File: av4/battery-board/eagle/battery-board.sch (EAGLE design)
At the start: 66 parts, among them J100 ROCKETNET-BATTERY-14, J101 87758-0216, J102 87758-0216, Q100 Si2343DS-T1, Q101 SI4435DDY, Q102 SI4435DDY, Q103 SI1023X, Q104 SI1023X, U100 BQ3060PW

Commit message: Latest battery boards notes, handing off to Michael for final polishing.
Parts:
- C101, C102, C105, C109, C111, C112, C113, C114: device rcl_custom:C-EU0402-B-NOSILK -> rcl_custom:C-EU0603-B-NOSILK
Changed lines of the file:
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@@
 <setting verticaltext="up"/>
 </settings>
-<grid distance="0.05" unitdist="inch" unit="inch" style="lines" multiple="2" display="yes" altdistance="0.01" altunitdist="inch" altunit="inch"/>
+<grid distance="0.1" unitdist="inch" unit="inch" style="lines" multiple="1" display="no" altdistance="0.01" altunitdist="inch" altunit="inch"/>
 <layers>
 <layer number="1" name="Top" color="4" fill="1" visible="no" active="no"/>
@@
 <part name="R120" library="rcl_custom" deviceset="R-US_" device="0603-B-NOSILK" value="100"/>
 <part name="R121" library="rcl_custom" deviceset="R-US_" device="0603-B-NOSILK" value="100"/>
-<part name="C111" library="rcl_custom" deviceset="C-EU" device="0402-B-NOSILK" value="100n"/>
-<part name="C113" library="rcl_custom" deviceset="C-EU" device="0402-B-NOSILK" value="100n"/>
-<part name="C112" library="rcl_custom" deviceset="C-EU" device="0402-B-NOSILK" value="100n"/>
+<part name="C111" library="rcl_custom" deviceset="C-EU" device="0603-B-NOSILK" value="100n"/>
+<part name="C113" library="rcl_custom" deviceset="C-EU" device="0603-B-NOSILK" value="100n"/>
+<part name="C112" library="rcl_custom" deviceset="C-EU" device="0603-B-NOSILK" value="100n"/>
 <part name="BAR_GND4" library="psas" deviceset="SUP_GND_BAR" device=""/>
 <part name="BAR_GND6" library="psas" deviceset="SUP_GND_BAR" device=""/>
@@
 <part name="R111" library="rcl_custom" deviceset="R-US_" device="0603-B-NOSILK" value="1K"/>
 <part name="R119" library="rcl_custom" deviceset="R-US_" device="0603-B-NOSILK" value="1K"/>
-<part name="C101" library="rcl_custom" deviceset="C-EU" device="0402-B-NOSILK" value="100n"/>
-<part name="C102" library="rcl_custom" deviceset="C-EU" device="0402-B-NOSILK" value="100n"/>
-<part name="C105" library="rcl_custom" deviceset="C-EU" device="0402-B-NOSILK" value="100n"/>
-<part name="C114" library="rcl_custom" deviceset="C-EU" device="0402-B-NOSILK" value="100n"/>
+<part name="C101" library="rcl_custom" deviceset="C-EU" device="0603-B-NOSILK" value="100n"/>
+<part name="C102" library="rcl_custom" deviceset="C-EU" device="0603-B-NOSILK" value="100n"/>
+<part name="C105" library="rcl_custom" deviceset="C-EU" device="0603-B-NOSILK" value="100n"/>
+<part name="C114" library="rcl_custom" deviceset="C-EU" device="0603-B-NOSILK" value="100n"/>
 <part name="BAR_GND8" library="psas" deviceset="SUP_GND_BAR" device=""/>
 <part name="BAR_GND9" library="psas" deviceset="SUP_GND_BAR" device=""/>
@@
 <part name="BAR_GND11" library="psas" deviceset="SUP_GND_BAR" device=""/>
 <part name="BAR_GND12" library="psas" deviceset="SUP_GND_BAR" device=""/>
-<part name="C109" library="rcl_custom" deviceset="C-EU" device="0402-B-NOSILK" value="100n"/>
+<part name="C109" library="rcl_custom" deviceset="C-EU" device="0603-B-NOSILK" value="100n"/>
 <part name="C110" library="rcl_custom" deviceset="C-EU" device="0603-B-NOSILK" value="1u"/>
 <part name="D101" library="diode-0603" deviceset="DIODE-0603" device=""/>

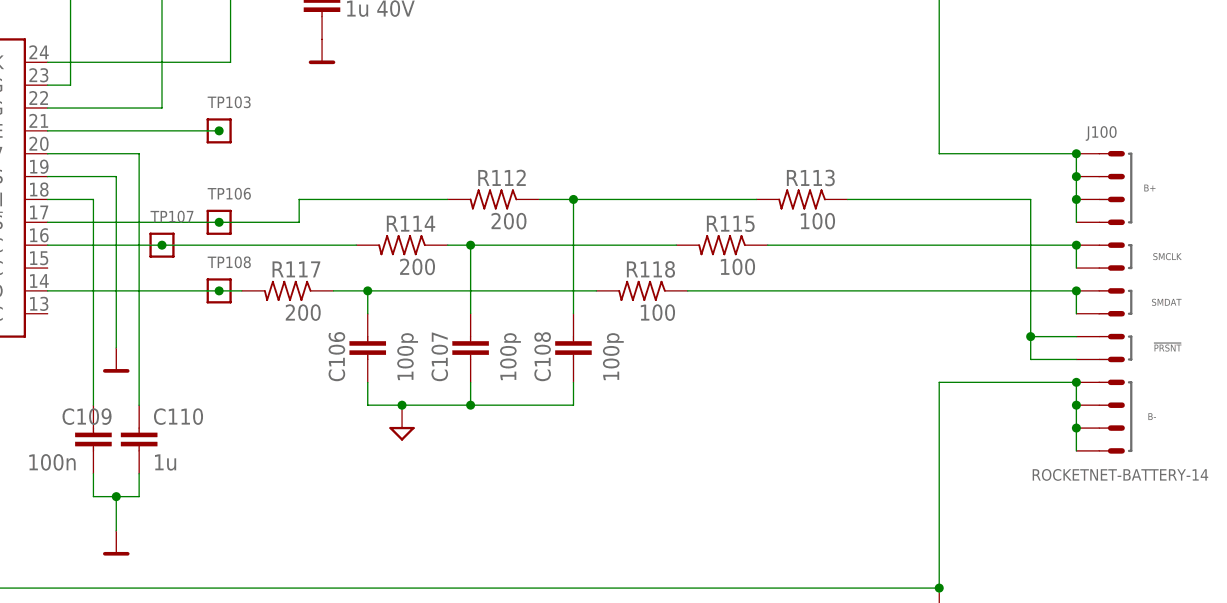
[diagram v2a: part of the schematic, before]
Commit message: moved some routing to top layer, needs drc work
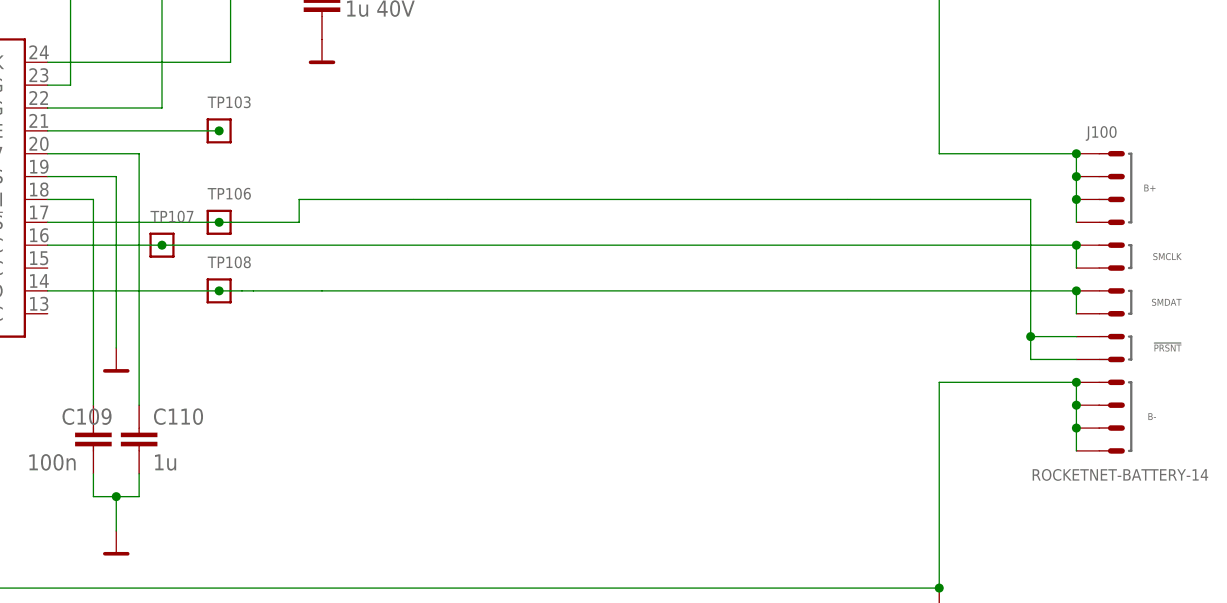
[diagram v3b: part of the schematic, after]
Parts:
- removed C106, C107, C108: 100p, rcl_custom:C-EU0603-B-NOSILK
- removed R112, R114, R117: 200, rcl_custom:R-US_0603-B-NOSILK
- removed R113, R115, R118: 100, rcl_custom:R-US_0603-B-NOSILK
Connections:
- removed net N$17: C106.1, R117.1, R118.2
- removed net N$24: C107.1, R114.1, R115.2
- removed net N$33: C108.1, R112.1, R113.2
- removed net RNC-!PRSNT: J100.!PRSNT@1, J100.!PRSNT@2, R113.1
- removed net RNC-SDAT: J100.SMDAT@1, J100.SMDAT@2, R118.1
- removed net SMBC: R114.2, TP107.P$1, U100.SMBC
- net !PRES: now also J100.!PRSNT@1, J100.!PRSNT@2; no longer R112.2
- net RNC-SCLK: now also TP107.P$1, U100.SMBC; no longer R115.1
- net SMBD: now also J100.SMDAT@1, J100.SMDAT@2; no longer R117.2
- net TRIANGLE_GND: no longer C106.2, C107.2, C108.2
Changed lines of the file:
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@@
 <part name="R110" library="rcl_custom" deviceset="R-US_" device="0603-B-NOSILK" value="100 .25W"/>
 <part name="R105" library="rcl_custom" deviceset="R-US_" device="0603-B-NOSILK" value="100 .25W"/>
-<part name="R114" library="rcl_custom" deviceset="R-US_" device="0603-B-NOSILK" value="200"/>
-<part name="R115" library="rcl_custom" deviceset="R-US_" device="0603-B-NOSILK" value="100"/>
-<part name="R117" library="rcl_custom" deviceset="R-US_" device="0603-B-NOSILK" value="200"/>
-<part name="R118" library="rcl_custom" deviceset="R-US_" device="0603-B-NOSILK" value="100"/>
-<part name="C106" library="rcl_custom" deviceset="C-EU" device="0603-B-NOSILK" value="100p"/>
-<part name="TRIANGLE_GND1" library="psas" deviceset="SUP_GND_TRIANGLE" device=""/>
-<part name="C107" library="rcl_custom" deviceset="C-EU" device="0603-B-NOSILK" value="100p"/>
 <part name="D102" library="diode-0603" deviceset="DIODE-0603" device=""/>
 <part name="C104" library="rcl_custom" deviceset="C-EU" device="0603-B-NOSILK" value="1u 40V"/>
 <part name="BAR_GND14" library="psas" deviceset="SUP_GND_BAR" device=""/>
-<part name="R112" library="rcl_custom" deviceset="R-US_" device="0603-B-NOSILK" value="200"/>
-<part name="R113" library="rcl_custom" deviceset="R-US_" device="0603-B-NOSILK" value="100"/>
-<part name="C108" library="rcl_custom" deviceset="C-EU" device="0603-B-NOSILK" value="100p"/>
 <part name="TRIANGLE_GND2" library="psas" deviceset="SUP_GND_TRIANGLE" device=""/>
 <part name="R108" library="rcl_custom" deviceset="R-US_" device="0603-B-NOSILK" value="5.1k"/>
@@
 <instance part="R110" gate="R" x="101.6" y="147.32" rot="MR90"/>
 <instance part="R105" gate="R" x="96.52" y="172.72" rot="MR90"/>
-<instance part="R114" gate="R" x="250.19" y="127" rot="MR0"/>
-<instance part="R115" gate="R" x="285.75" y="127" rot="MR0"/>
-<instance part="R117" gate="R" x="237.49" y="121.92" rot="MR0"/>
-<instance part="R118" gate="R" x="276.86" y="121.92" rot="MR0"/>
-<instance part="C106" gate="CE" x="246.38" y="116.84" smashed="yes">
-<attribute name="NAME" x="243.84" y="111.76" size="1.778" layer="95" rot="R90"/>
-<attribute name="VALUE" x="251.46" y="111.76" size="1.778" layer="96" rot="R90"/>
-</instance>
-<instance part="TRIANGLE_GND1" gate="1" x="250.19" y="106.68" smashed="yes"/>
-<instance part="C107" gate="CE" x="257.81" y="116.84" smashed="yes">
-<attribute name="NAME" x="255.27" y="111.76" size="1.778" layer="95" rot="R90"/>
-<attribute name="VALUE" x="262.89" y="111.76" size="1.778" layer="96" rot="R90"/>
-</instance>
 <instance part="D102" gate="G$1" x="241.3" y="165.1" rot="R90"/>
 <instance part="C104" gate="CE" x="241.3" y="154.94" smashed="yes">
@@
 </instance>
 <instance part="BAR_GND14" gate="1" x="241.3" y="147.32" smashed="yes"/>
-<instance part="R112" gate="R" x="260.35" y="132.08" rot="MR0"/>
-<instance part="R113" gate="R" x="294.64" y="132.08" rot="MR0"/>
-<instance part="C108" gate="CE" x="269.24" y="116.84" smashed="yes">
-<attribute name="NAME" x="266.7" y="111.76" size="1.778" layer="95" rot="R90"/>
-<attribute name="VALUE" x="274.32" y="111.76" size="1.778" layer="96" rot="R90"/>
-</instance>
 <instance part="TRIANGLE_GND2" gate="1" x="261.62" y="175.26" smashed="yes"/>
 <instance part="R108" gate="R" x="223.52" y="167.64" rot="MR270"/>
@@
 <pinref part="C110" gate="CE" pin="1"/>
 <pinref part="U100" gate="G$1" pin="REG27"/>
-</segment>
-</net>
-<net name="SMBD" class="0">
-<segment>
-<wire x1="210.82" y1="121.92" x2="229.87" y2="121.92" width="0.1524" layer="91"/>
-<pinref part="U100" gate="G$1" pin="SMBD"/>
-<pinref part="R117" gate="R" pin="2"/>
-<pinref part="TP108" gate="G$1" pin="P$1"/>
-<junction x="229.87" y="121.92"/>
-<wire x1="229.87" y1="121.92" x2="232.41" y2="121.92" width="0.1524" layer="91"/>
-</segment>
-</net>
-<net name="SMBC" class="0">
-<segment>
-<wire x1="210.82" y1="127" x2="223.52" y2="127" width="0.1524" layer="91"/>
-<wire x1="223.52" y1="127" x2="245.11" y2="127" width="0.1524" layer="91"/>
-<junction x="223.52" y="127"/>
-<pinref part="U100" gate="G$1" pin="SMBC"/>
-<pinref part="R114" gate="R" pin="2"/>
-<pinref part="TP107" gate="G$1" pin="P$1"/>
 </segment>
 </net>
@@
 </segment>
 <segment>
-<wire x1="269.24" y1="109.22" x2="257.81" y2="109.22" width="0.1524" layer="91"/>
-<wire x1="257.81" y1="109.22" x2="257.81" y2="111.76" width="0.1524" layer="91"/>
-<wire x1="250.19" y1="109.22" x2="246.38" y2="109.22" width="0.1524" layer="91"/>
-<wire x1="246.38" y1="109.22" x2="246.38" y2="111.76" width="0.1524" layer="91"/>
-<wire x1="250.19" y1="109.22" x2="257.81" y2="109.22" width="0.1524" layer="91"/>
-<junction x="257.81" y="109.22"/>
-<junction x="250.19" y="109.22"/>
-<pinref part="C107" gate="CE" pin="2"/>
-<pinref part="C106" gate="CE" pin="2"/>
-<pinref part="TRIANGLE_GND1" gate="1" pin="TRIANGLE_GND"/>
-<pinref part="C108" gate="CE" pin="2"/>
-<wire x1="269.24" y1="111.76" x2="269.24" y2="109.22" width="0.1524" layer="91"/>
-</segment>
-<segment>
 <wire x1="261.62" y1="180.34" x2="261.62" y2="177.8" width="0.1524" layer="91"/>
 <pinref part="TRIANGLE_GND2" gate="1" pin="TRIANGLE_GND"/>
@@
 </segment>
 </net>
-<net name="N$17" class="0">
-<segment>
-<wire x1="242.57" y1="121.92" x2="246.38" y2="121.92" width="0.1524" layer="91"/>
-<wire x1="246.38" y1="121.92" x2="271.78" y2="121.92" width="0.1524" layer="91"/>
-<wire x1="246.38" y1="119.38" x2="246.38" y2="121.92" width="0.1524" layer="91"/>
-<junction x="246.38" y="121.92"/>
-<pinref part="R117" gate="R" pin="1"/>
-<pinref part="R118" gate="R" pin="2"/>
-<pinref part="C106" gate="CE" pin="1"/>
-</segment>
-</net>
-<net name="RNC-SDAT" class="0">
-<segment>
-<wire x1="281.94" y1="121.92" x2="325.12" y2="121.92" width="0.1524" layer="91"/>
-<pinref part="R118" gate="R" pin="1"/>
-<pinref part="J100" gate="G$1" pin="SMDAT@2"/>
-<wire x1="325.12" y1="119.38" x2="325.12" y2="121.92" width="0.1524" layer="91"/>
-<pinref part="J100" gate="G$1" pin="SMDAT@1"/>
-<junction x="325.12" y="121.92"/>
-</segment>
-</net>
-<net name="N$24" class="0">
-<segment>
-<wire x1="255.27" y1="127" x2="257.81" y2="127" width="0.1524" layer="91"/>
-<wire x1="257.81" y1="127" x2="280.67" y2="127" width="0.1524" layer="91"/>
-<wire x1="257.81" y1="119.38" x2="257.81" y2="127" width="0.1524" layer="91"/>
-<junction x="257.81" y="127"/>
-<pinref part="R114" gate="R" pin="1"/>
-<pinref part="R115" gate="R" pin="2"/>
-<pinref part="C107" gate="CE" pin="1"/>
-</segment>
-</net>
 <net name="RNC-SCLK" class="0">
 <segment>
-<wire x1="290.83" y1="127" x2="325.12" y2="127" width="0.1524" layer="91"/>
-<pinref part="R115" gate="R" pin="1"/>
 <pinref part="J100" gate="G$1" pin="SMCLK@2"/>
 <wire x1="325.12" y1="124.46" x2="325.12" y2="127" width="0.1524" layer="91"/>
 <pinref part="J100" gate="G$1" pin="SMCLK@1"/>
 <junction x="325.12" y="127"/>
+<wire x1="210.82" y1="127" x2="223.52" y2="127" width="0.1524" layer="91"/>
+<junction x="223.52" y="127"/>
+<pinref part="U100" gate="G$1" pin="SMBC"/>
+<pinref part="TP107" gate="G$1" pin="P$1"/>
+<wire x1="325.12" y1="127" x2="223.52" y2="127" width="0.1524" layer="91"/>
 </segment>
 </net>
@@
 <wire x1="229.87" y1="129.54" x2="238.76" y2="129.54" width="0.1524" layer="91"/>
 <wire x1="238.76" y1="129.54" x2="238.76" y2="132.08" width="0.1524" layer="91"/>
-<wire x1="238.76" y1="132.08" x2="255.27" y2="132.08" width="0.1524" layer="91"/>
+<wire x1="238.76" y1="132.08" x2="251.46" y2="132.08" width="0.1524" layer="91"/>
 <junction x="229.87" y="129.54"/>
 <pinref part="U100" gate="G$1" pin="!PRES"/>
-<pinref part="R112" gate="R" pin="2"/>
 <pinref part="TP106" gate="G$1" pin="P$1"/>
-</segment>
-</net>
-<net name="N$33" class="0">
-<segment>
-<wire x1="265.43" y1="132.08" x2="269.24" y2="132.08" width="0.1524" layer="91"/>
-<wire x1="269.24" y1="132.08" x2="289.56" y2="132.08" width="0.1524" layer="91"/>
-<wire x1="269.24" y1="132.08" x2="269.24" y2="119.38" width="0.1524" layer="91"/>
-<junction x="269.24" y="132.08"/>
-<pinref part="R112" gate="R" pin="1"/>
-<pinref part="R113" gate="R" pin="2"/>
-<pinref part="C108" gate="CE" pin="1"/>
-</segment>
-</net>
-<net name="RNC-!PRSNT" class="0">
-<segment>
-<wire x1="299.72" y1="132.08" x2="320.04" y2="132.08" width="0.1524" layer="91"/>
-<pinref part="R113" gate="R" pin="1"/>
+<wire x1="251.46" y1="132.08" x2="255.27" y2="132.08" width="0.1524" layer="91"/>
+<wire x1="299.72" y1="132.08" x2="302.26" y2="132.08" width="0.1524" layer="91"/>
+<wire x1="302.26" y1="132.08" x2="320.04" y2="132.08" width="0.1524" layer="91"/>
 <wire x1="320.04" y1="132.08" x2="320.04" y2="116.84" width="0.1524" layer="91"/>
 <pinref part="J100" gate="G$1" pin="!PRSNT@1"/>
@@
 <wire x1="320.04" y1="114.3" x2="320.04" y2="116.84" width="0.1524" layer="91"/>
 <junction x="320.04" y="116.84"/>
+<wire x1="255.27" y1="132.08" x2="299.72" y2="132.08" width="0.1524" layer="91"/>
 </segment>
 </net>
@@
 </segment>
 </net>
+<net name="SMBD" class="0">
+<segment>
+<pinref part="J100" gate="G$1" pin="SMDAT@2"/>
+<wire x1="325.12" y1="119.38" x2="325.12" y2="121.92" width="0.1524" layer="91"/>
+<pinref part="J100" gate="G$1" pin="SMDAT@1"/>
+<junction x="325.12" y="121.92"/>
+<wire x1="233.68" y1="121.92" x2="241.3" y2="121.92" width="0.1524" layer="91"/>
+<wire x1="241.3" y1="121.92" x2="325.12" y2="121.92" width="0.1524" layer="91"/>
+<wire x1="210.82" y1="121.92" x2="229.87" y2="121.92" width="0.1524" layer="91"/>
+<pinref part="U100" gate="G$1" pin="SMBD"/>
+<pinref part="TP108" gate="G$1" pin="P$1"/>
+<junction x="229.87" y="121.92"/>
+<wire x1="229.87" y1="121.92" x2="231.14" y2="121.92" width="0.1524" layer="91"/>
+<wire x1="231.14" y1="121.92" x2="232.41" y2="121.92" width="0.1524" layer="91"/>
+<wire x1="233.68" y1="121.92" x2="232.41" y2="121.92" width="0.1524" layer="91"/>
+</segment>
+</net>
